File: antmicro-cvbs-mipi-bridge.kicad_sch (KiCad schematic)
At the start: 105 parts, among them IC1 ADV7280BCPZ-M, IC2 TLV70018, IC4 SN74AUP1G17DCKR, IC5 SN74AUP1G17DCKR, J1 WE_68715014522, J2 61300211121, J7 61300211121, Q2 BSS138APW, Y1 ABM8G-28.63636MHZ-18-D2Y-T

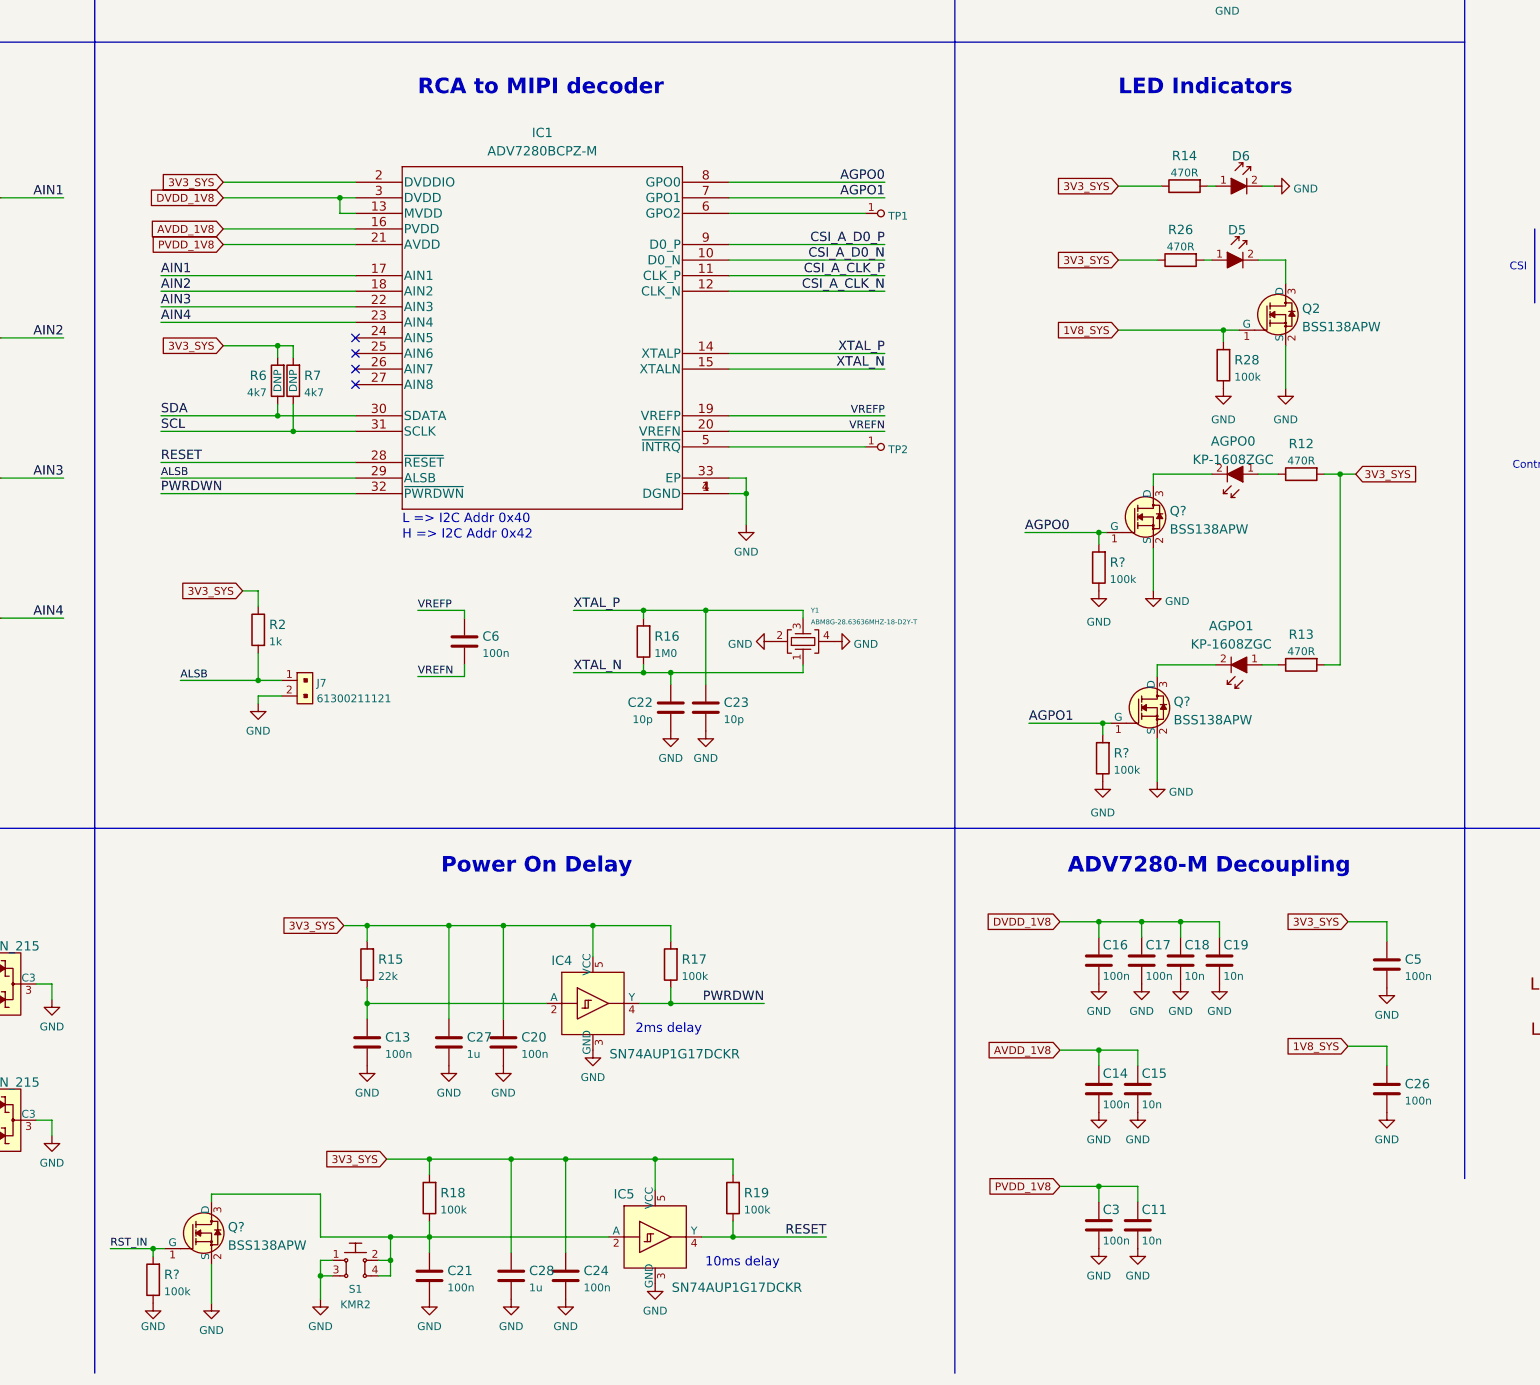
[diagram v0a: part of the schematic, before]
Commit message: Fixes adjusted visually. New components annotated
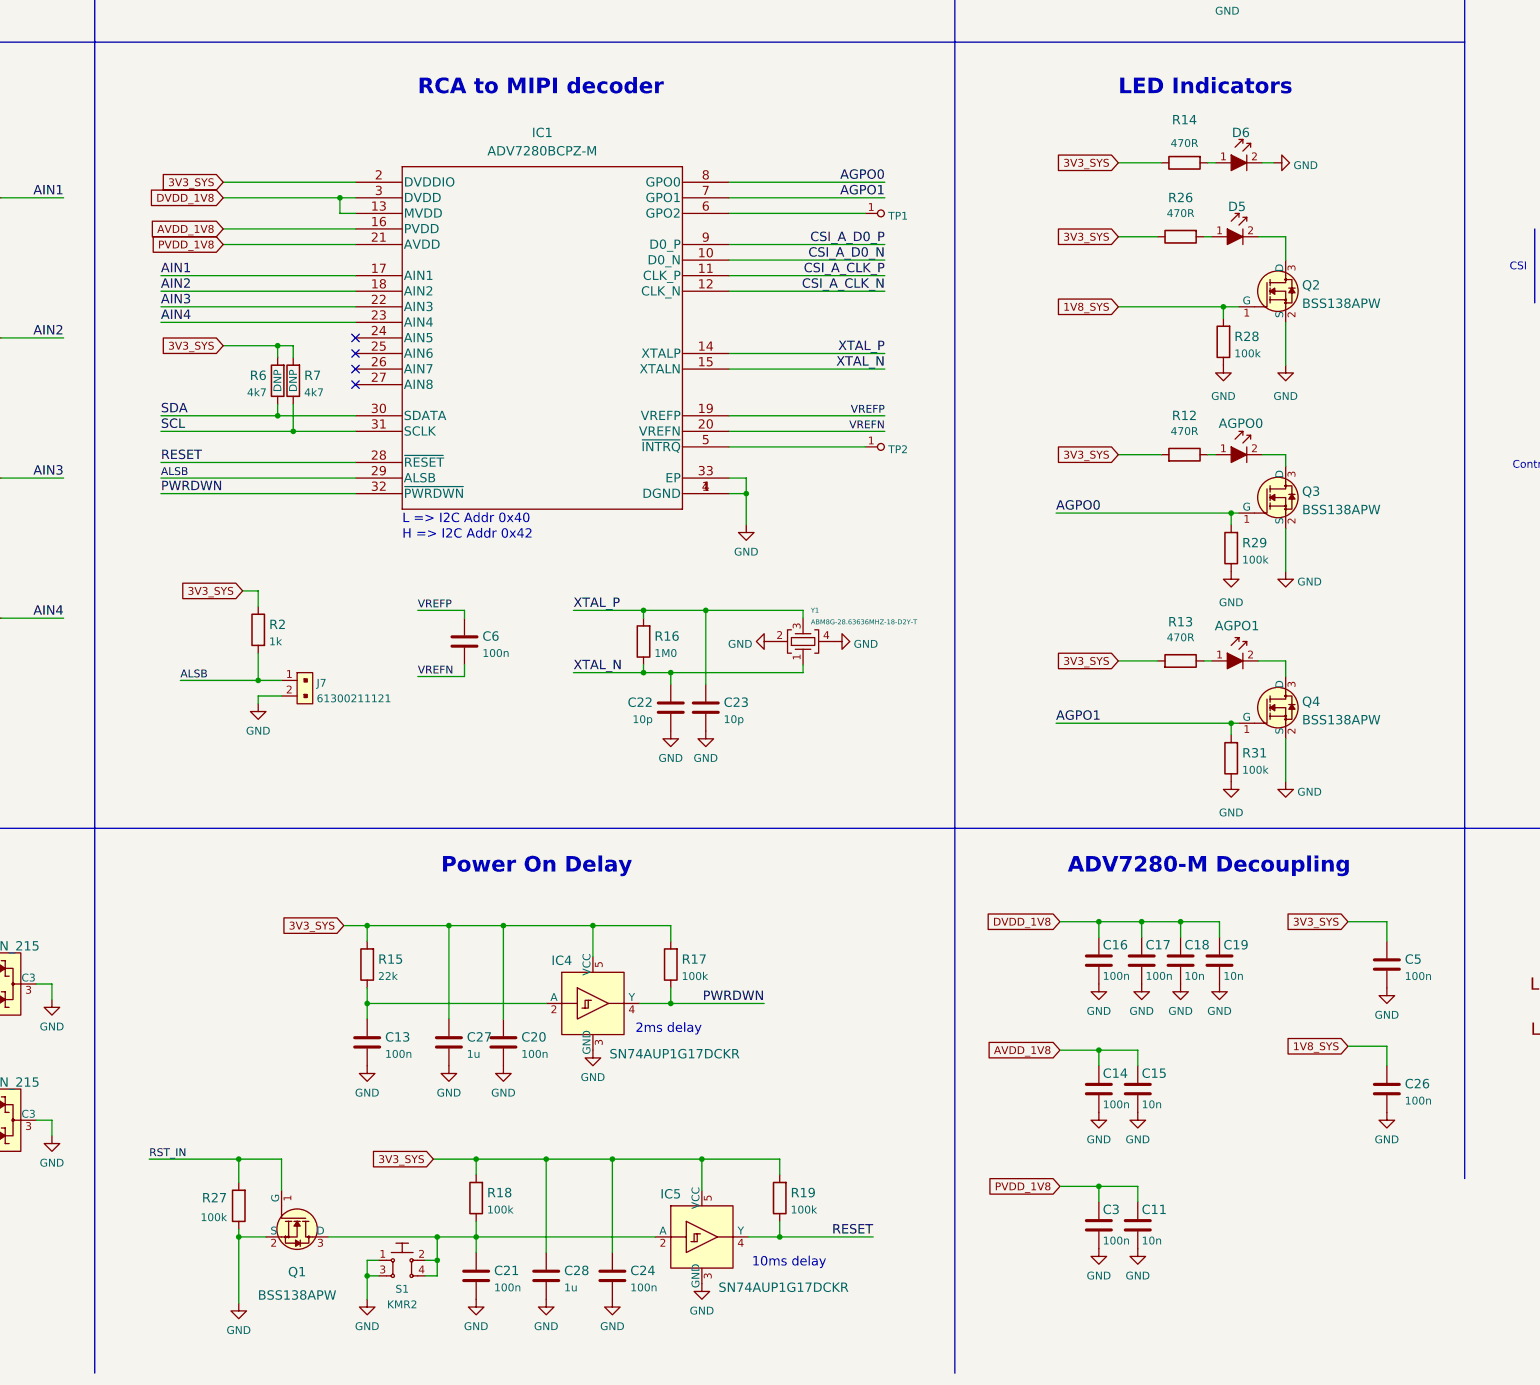
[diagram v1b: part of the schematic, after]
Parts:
- gave numbers to parts that had none: 6
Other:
- moved on the sheet: AGPO0, AGPO1, C21, C24, C28, D5, D6, IC5, Q1, Q2, Q3, Q4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
